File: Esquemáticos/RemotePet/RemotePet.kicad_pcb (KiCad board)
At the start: 2 copper layers, 87.2 x 72.6 mm, 28 parts, among them U1 ESP32_DevKit_V1_DOIT, U2 xfw-hx711, U4 LM1117-3.3, U5 L7805, U6 GY-30

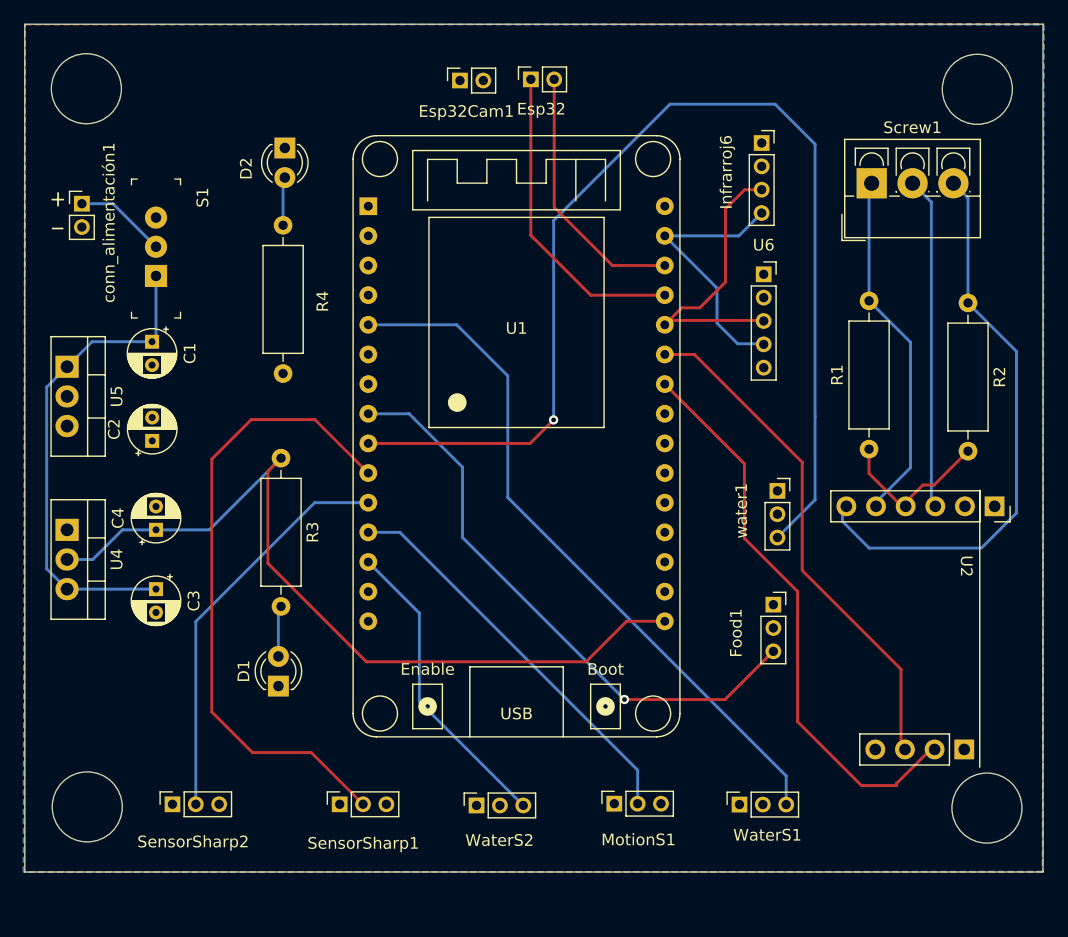
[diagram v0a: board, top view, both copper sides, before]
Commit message: PCB 2.0
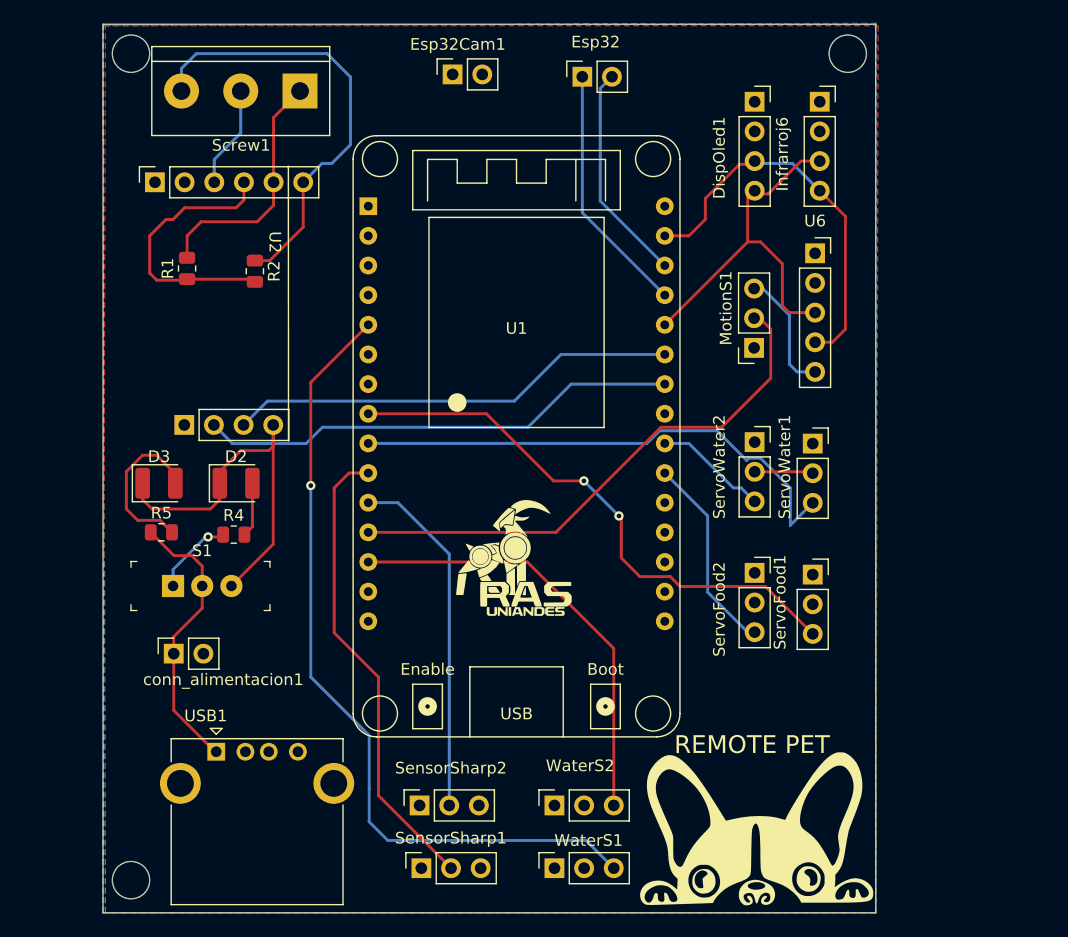
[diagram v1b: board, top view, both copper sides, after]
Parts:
- removed C1, C2: 0.22 uF, Capacitor_THT:CP_Radial_D4.0mm_P2.00mm
- removed C3, C4: 10uF, Capacitor_THT:CP_Radial_D4.0mm_P2.00mm
- removed D1: LED, LED_THT:LED_D3.0mm_Clear
- removed R3: 1KΩ, Resistor_THT:R_Axial_DIN0309_L9.0mm_D3.2mm_P12.70mm_Horizontal
- removed U4: LM1117-3.3, Package_TO_SOT_THT:TO-220-3_Vertical
- removed U5: L7805, Package_TO_SOT_THT:TO-220-3_Vertical
- removed conn_alimentación1: Conn_01x02_Male, Connector_PinHeader_2.00mm:PinHeader_1x02_P2.00mm_Vertical
- added D3: LED, LED_SMD:LED_1210_3225Metric, F.Cu at (104.4, 93.8)
- added DispOled1: Display 1, Connector_PinSocket_2.54mm:PinSocket_1x04_P2.54mm_Vertical, F.Cu at (155.4, 61.1)
- added G***: LOGO, RAS:RAS, F.Cu at (135.1, 100.9)
- added R5: 330Ω, Resistor_SMD:R_0805_2012Metric, F.Cu at (104.6, 98.0)
- added REMOTE PET: LOGO, Audio_Module:Perro, F.Cu at (155.6, 123.4)
- added ServoFood2: Servo3, Connector_PinSocket_2.54mm:PinSocket_1x03_P2.54mm_Vertical, F.Cu at (155.4, 101.5)
- added ServoWater2: Servo4, Connector_PinSocket_2.54mm:PinSocket_1x03_P2.54mm_Vertical, F.Cu at (155.4, 90.3)
- added USB1: USB_A, Connector_USB:USB_A_CONNFLY_DS1095-WNR0, F.Cu at (109.3, 116.8)
- added conn_alimentacion1: Conn_01x02_Male, Connector_PinSocket_2.54mm:PinSocket_1x02_P2.54mm_Vertical, F.Cu at (105.7, 108.4)
- D2: footprint LED_THT:LED_D3.0mm_Clear -> LED_SMD:LED_1210_3225Metric
- Esp32, Esp32Cam1: footprint Connector_PinSocket_2.00mm:PinSocket_1x02_P2.00mm_Vertical -> Connector_PinSocket_2.54mm:PinSocket_1x02_P2.54mm_Vertical
- Infrarroj6: footprint Connector_PinSocket_2.00mm:PinSocket_1x04_P2.00mm_Vertical -> Connector_PinSocket_2.54mm:PinSocket_1x04_P2.54mm_Vertical
- MotionS1, SensorSharp1, SensorSharp2, WaterS1, WaterS2: footprint Connector_PinSocket_2.00mm:PinSocket_1x03_P2.00mm_Vertical -> Connector_PinSocket_2.54mm:PinSocket_1x03_P2.54mm_Vertical
- R1, R2: footprint Resistor_THT:R_Axial_DIN0309_L9.0mm_D3.2mm_P12.70mm_Horizontal -> Resistor_SMD:R_0805_2012Metric
- R4: value 1KΩ -> 330Ω; footprint Resistor_THT:R_Axial_DIN0309_L9.0mm_D3.2mm_P12.70mm_Horizontal -> Resistor_SMD:R_0805_2012Metric
- Screw1: footprint TerminalBlock_4Ucon:TerminalBlock_4Ucon_1x03_P3.50mm_Vertical -> TerminalBlock:TerminalBlock_bornier-3_P5.08mm
- ServoFood1: renamed from Food1; footprint Connector_PinSocket_2.00mm:PinSocket_1x03_P2.00mm_Vertical -> Connector_PinSocket_2.54mm:PinSocket_1x03_P2.54mm_Vertical
- ServoWater1: renamed from water1; footprint Connector_PinSocket_2.00mm:PinSocket_1x03_P2.00mm_Vertical -> Connector_PinSocket_2.54mm:PinSocket_1x03_P2.54mm_Vertical
- U6: footprint Connector_PinSocket_2.00mm:PinSocket_1x05_P2.00mm_Vertical -> Connector_PinSocket_2.54mm:PinSocket_1x05_P2.54mm_Vertical
- moved U2 65.4 mm to (114.4, 88.9)
- moved R2 61.2 mm to (112.6, 75.6)
- moved R1 60.4 mm to (106.8, 75.4)
- moved Screw1 49.6 mm to (116.5, 60.2), turned to 180 degrees
- moved MotionS1 40.8 mm to (155.4, 82.2), turned to 180 degrees
- moved D2 29.0 mm to (111.0, 93.8), turned to 0 degrees
- moved S1 26.6 mm to (105.6, 102.6), turned to 0 degrees
- moved SensorSharp2 21.2 mm to (126.7, 121.4)
- moved WaterS1 16.8 mm to (138.3, 126.8)
- moved R4 14.4 mm to (110.8, 98.2), turned to 0 degrees
- moved SensorSharp1 8.89 mm to (126.9, 126.8)
- moved WaterS2 6.68 mm to (138.3, 121.4)
- moved Infrarroj6 6.10 mm to (161.0, 61.1)
- moved ServoWater1 5.06 mm to (160.4, 90.4)
- moved U6 4.75 mm to (160.6, 74.1)
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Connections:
- S1 pad 1: VCC -> 5V
- S1 pad 2: Net-(S1-Pad2) -> VCC
- U1 pad 21: unconnected-(U1-Pad21) -> IO16
- U1 pad 22: unconnected-(U1-Pad22) -> IO17
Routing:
- net 3.3V: track 70.3 -> 0.00 mm
- net IO26: track 96.8 -> 44.7 mm, vias 1 -> 0
- net GND: track 0.00 -> 38.7 mm
- net Net-(Screw1-Pad2): track 28.3 -> 8.76 mm
- net VCC: track 42.1 -> 24.1 mm
- net 5V: track 0.00 -> 16.8 mm, vias 0 -> 1
- net IO16: track 0.00 -> 16.6 mm
- net IO27: track 54.6 -> 40.2 mm
- net Net-(R5-Pad2): track 0.00 -> 14.2 mm
- net IO13: track 26.4 -> 37.5 mm
- net IO12: track 34.4 -> 45.5 mm
- net IO22: track 23.1 -> 34.0 mm
- net Net-(R2-Pad1): track 48.9 -> 38.1 mm
- net Net-(R1-Pad1): track 13.7 -> 23.4 mm
- net IO17: track 0.00 -> 9.76 mm
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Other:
- board size 87.2 x 72.6 mm -> 66.2 x 76.1 mm
- board text added: "Screw_Terminal_01x03"
